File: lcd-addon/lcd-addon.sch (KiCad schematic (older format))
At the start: 8 parts, among them J1 Conn_01x02_Male, J2 Conn_01x07_Male, J4 Conn_01x10, J5 Conn_01x01_Male, J6 Conn_01x02_Male, J8 Conn_01x02_Male

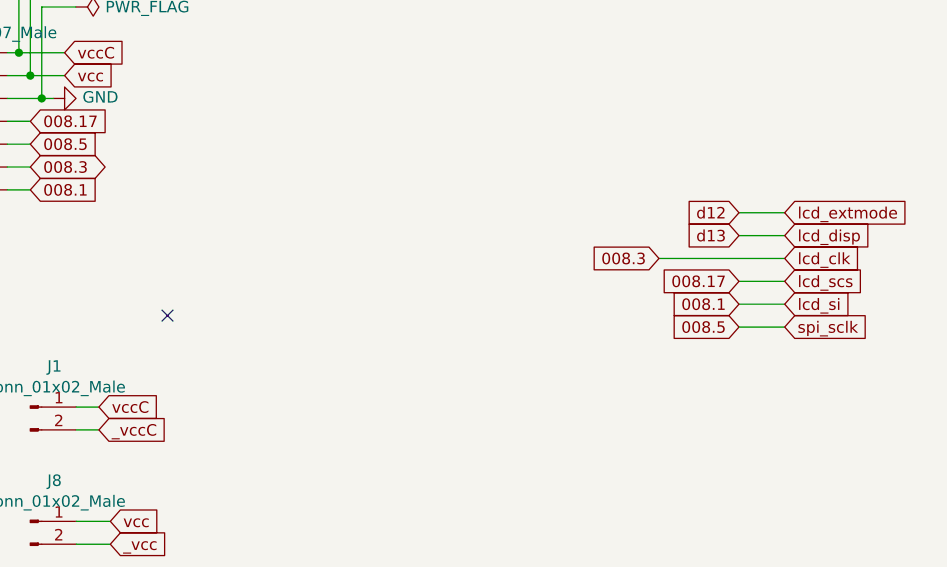
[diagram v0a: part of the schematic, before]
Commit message: lcd-addon changes
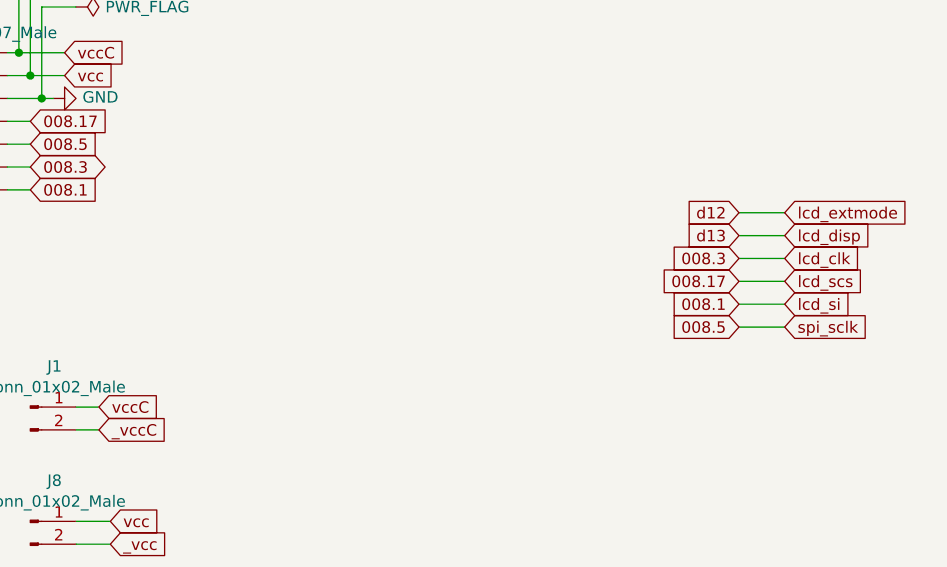
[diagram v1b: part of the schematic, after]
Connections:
- no-connect marks 2 -> 1
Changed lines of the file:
@@
 	-1   0    0    1
 $EndComp
-Text GLabel 5650 3650 0    50   Input ~ 0
+Text GLabel 6000 3650 0    50   Input ~ 0
 008.3
 Text GLabel 3250 4900 2    50   Input ~ 0
@@
 	3200 4400 3100 4400
 NoConn ~ 3050 6150
-NoConn ~ 3500 3900
 Wire Wire Line
-	5650 3650 6200 3650
+	6000 3650 6200 3650
 $EndSCHEMATC
